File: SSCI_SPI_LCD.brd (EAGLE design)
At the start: 110 x 100 mm, 33 parts, among them IC3 74LVC541_RGY, X1 PHA-1X08SG, X2 PHA-1X08SG

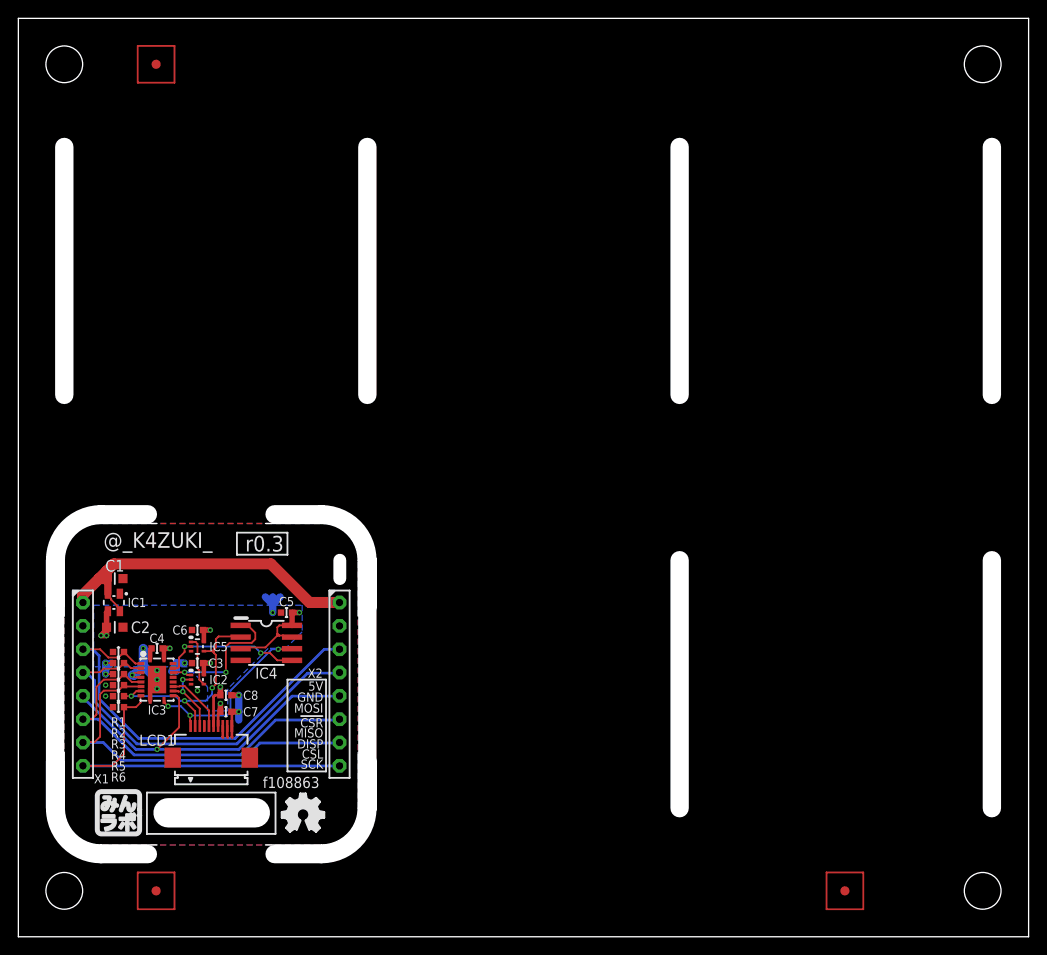
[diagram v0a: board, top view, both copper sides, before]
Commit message: 8c37b00 panelized
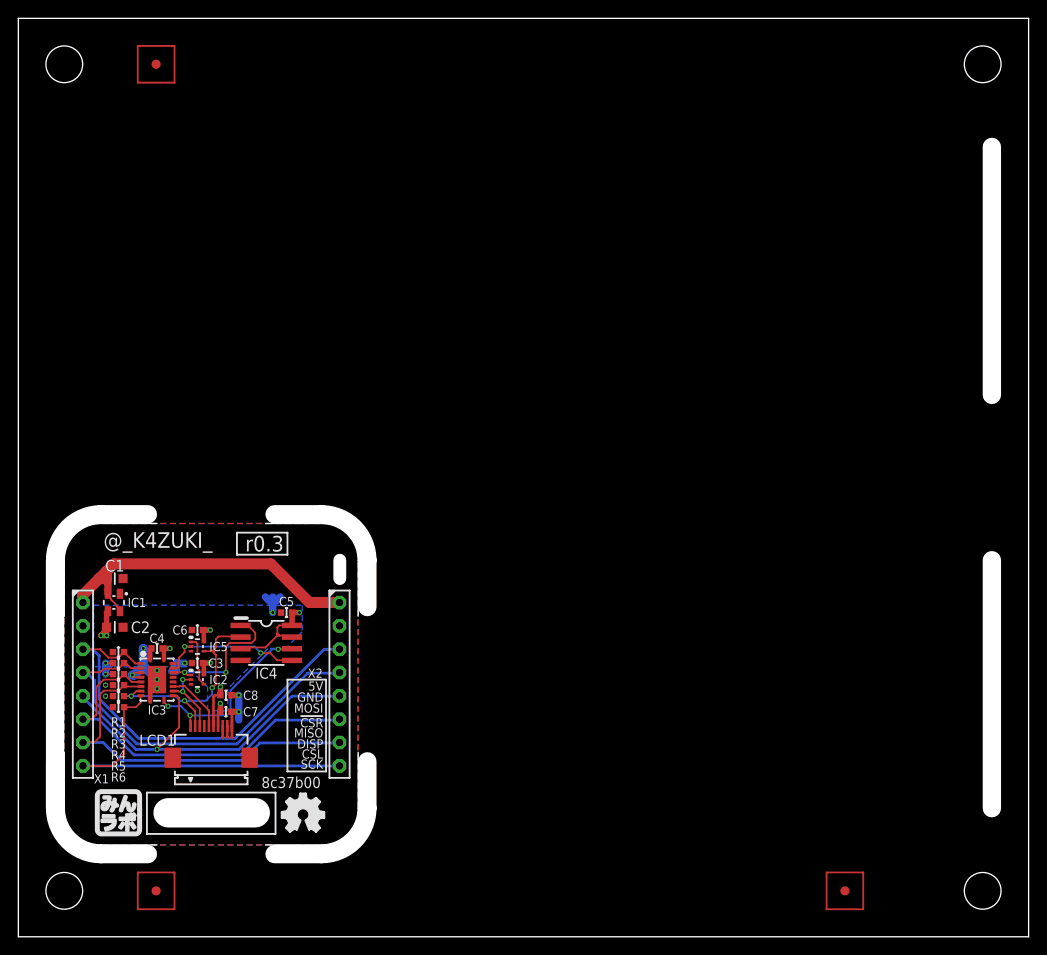
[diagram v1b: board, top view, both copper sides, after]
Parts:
- GIT1: value f108863 -> 8c37b00
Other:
- outline, holes or cut-outs redrawn
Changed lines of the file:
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@@
 <dimension x1="110" y1="0" x2="105" y2="0" x3="107.5" y3="-6.9" textsize="1.778" layer="47"/>
 <rectangle x1="5" y1="10" x2="37" y2="45" layer="37"/>
-<wire x1="38" y1="14" x2="38" y2="41" width="2" layer="46"/>
-<wire x1="38" y1="59" x2="38" y2="86" width="2" layer="46"/>
-<wire x1="72" y1="59" x2="72" y2="86" width="2" layer="46"/>
-<wire x1="72" y1="14" x2="72" y2="41" width="2" layer="46"/>
+<wire x1="38" y1="14" x2="38" y2="41" width="2" layer="51"/>
+<wire x1="38" y1="59" x2="38" y2="86" width="2" layer="51"/>
+<wire x1="72" y1="59" x2="72" y2="86" width="2" layer="51"/>
+<wire x1="72" y1="14" x2="72" y2="41" width="2" layer="51"/>
 <wire x1="106" y1="14" x2="106" y2="41" width="2" layer="46"/>
 <wire x1="106" y1="59" x2="106" y2="86" width="2" layer="46"/>
-<wire x1="5" y1="59" x2="5" y2="86" width="2" layer="46"/>
+<wire x1="4" y1="59" x2="4" y2="86" width="2" layer="51"/>
 <wire x1="35" y1="41" x2="35" y2="39" width="1.4" layer="46"/>
 <wire x1="35" y1="41" x2="35" y2="39" width="2" layer="41"/>
@@
 <attribute name="NOT_COMPONENT" value="YES" x="9" y="14" size="1.778" layer="27" rot="R270" display="off"/>
 </element>
-<element name="GIT1" library="git-revision" package="GIT-REVISION_1.2" value="f108863" x="29.7" y="16.8">
+<element name="GIT1" library="git-revision" package="GIT-REVISION_1.2" value="8c37b00" x="29.7" y="16.8">
 <attribute name="NOT_COMPONENT" value="YES" x="29.7" y="16.8" size="1.778" layer="27" display="off"/>
 </element>
